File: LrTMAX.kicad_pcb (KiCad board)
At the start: 4 copper layers, 100 x 100 mm, 126 parts, among them J1 USB_C_Receptacle_USB2.0, J2 Conn_02x05_Odd_Even, Q1 2N7002, SW1 Tact_SW_8mm, SW10 EC11_SMD, SW11 EC11_SMD, SW12 EC11_SMD, SW13 EC11_SMD, SW14 EC11_SMD, SW15 EC11_SMD, SW16 EC11_SMD, SW17 EC11_SMD, SW2 Tact_SW_8mm, SW20 SW_SPST, SW3 Tact_SW_8mm, SW4 Tact_SW_8mm, SW5 Tact_SW_8mm, SW6 Tact_SW_8mm, SW7 Tact_SW_8mm, SW8 Tact_SW_8mm, U1 STM32F072C8Tx, U3 SSD1306_OLED_0.91, U4 SPX3819M5-L3-3TR

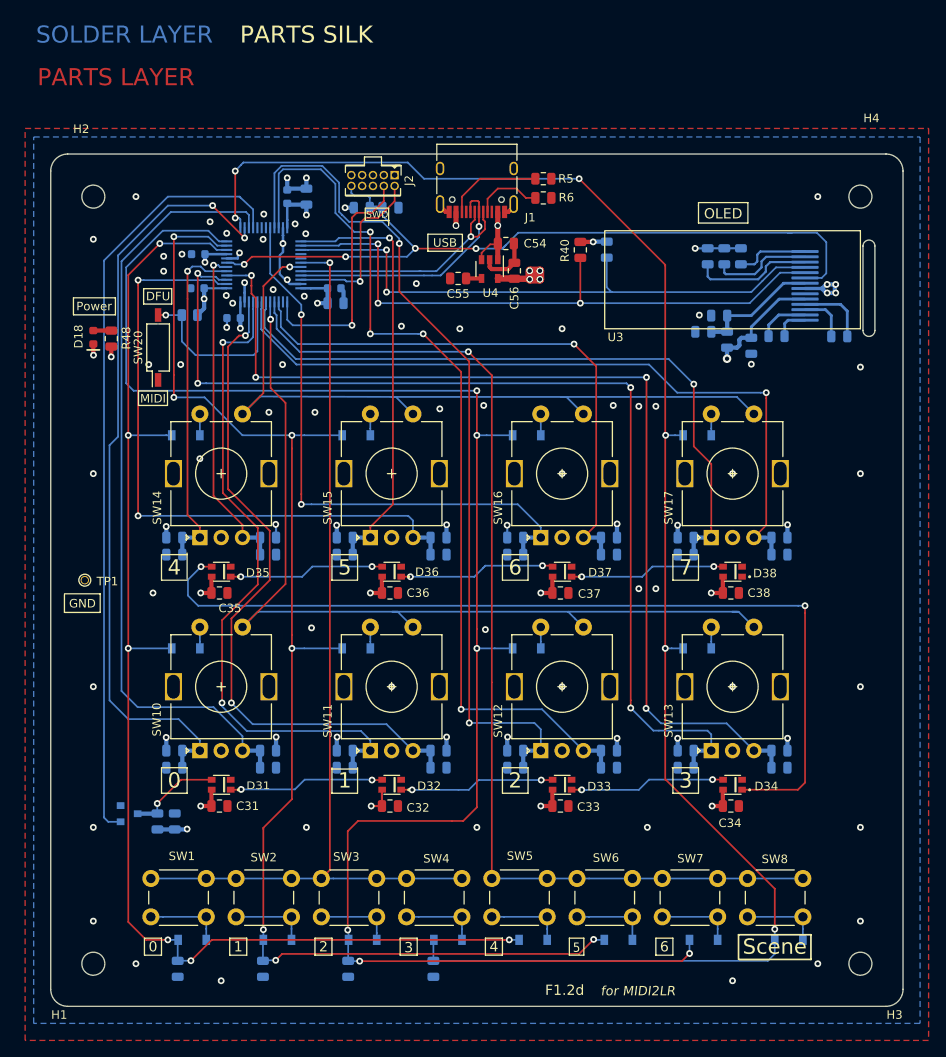
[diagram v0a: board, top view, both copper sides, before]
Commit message: trace drawn except CPU.
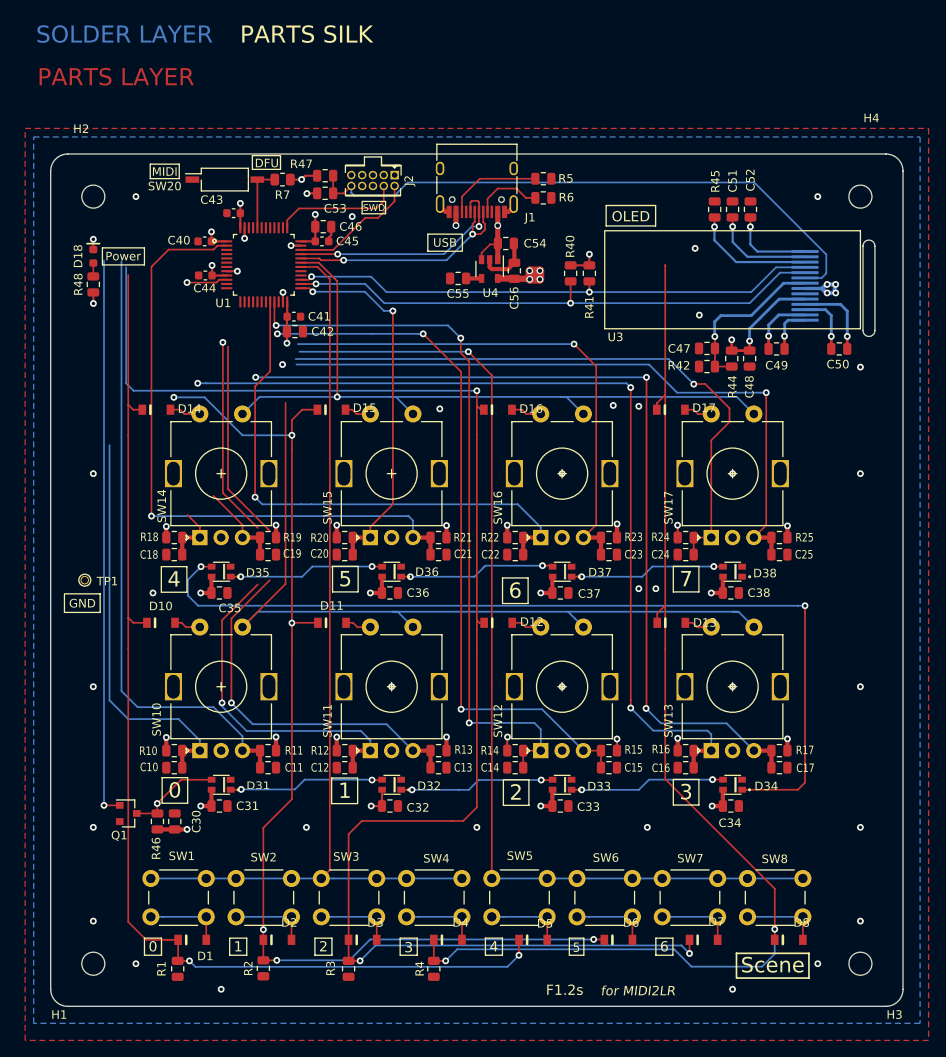
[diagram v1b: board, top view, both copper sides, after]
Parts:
- C10, C11, C12, C13, C14, C15, C16, C17, C18, C19, C20, C21, C22, C23, C24, C25, C30, C40, C41, C42, C43, C44, C45, C46, C47, C48, C49, C50, C51, C52, C53, D1, D10, D11, D12, D13, D14, D15, D16, D17, D2, D3, D4, D5, D6, D7, D8, Q1, R1, R10, R11, R12, R13, R14, R15, R16, R17, R18, R19, R2, R20, R21, R22, R23, R24, R25, R3, R4, R41, R42, R44, R45, R46, R47, R7, U1: moved to F.Cu
- moved SW20 21.2 mm to (120.4, 103.0), turned to 0 degrees
- moved R7 19.3 mm to (127.2, 103.0)
- moved C42 15.9 mm to (128.7, 120.8), turned to 180 degrees
- moved C41 14.1 mm to (128.5, 119.1), turned to 180 degrees
- moved C43 12.3 mm to (121.5, 106.9)
- moved D18 9.50 mm to (105.0, 112.0), turned to -90 degrees
- moved C46 9.08 mm to (132.0, 108.5)
- moved C53 7.85 mm to (132.2, 104.6), turned to 180 degrees
- moved R48 6.70 mm to (105.0, 115.3)
- moved R47 5.71 mm to (132.2, 102.5)
- moved C45 5.68 mm to (131.8, 110.2)
- moved C52 5.61 mm to (182.1, 106.5)
- moved C51 5.58 mm to (180.0, 106.5)
- moved C40 5.57 mm to (118.1, 110.2)
- moved R45 5.56 mm to (177.9, 106.5)
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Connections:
- net Net-(R7-Pad2) renamed /DFU
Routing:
- net /M3: track 196.4 -> 136.4 mm, vias 6 -> 2
- net /ENC0A: track 90.4 -> 47.7 mm, vias 2 -> 0
- net /ENC4A: track 41.0 -> 7.32 mm, vias 1 -> 0
- net /M1: track 157.2 -> 128.1 mm, vias 7 -> 6
- net /ENC4B: track 39.1 -> 10.4 mm, vias 1 -> 0
- net /LED_DON: track 90.9 -> 65.7 mm, vias 0 -> 1
- net /ENC2B: track 106.8 -> 83.4 mm, vias 4 -> 3
- net /NRST: track 92.3 -> 70.3 mm, vias 4 -> 0
- net /M2: track 200.1 -> 179.9 mm, vias 6 -> 3
- net /ENC0B: track 91.6 -> 72.6 mm
- net GND: track 45.8 -> 27.1 mm, vias 72 -> 43
- net /ENC3A: track 121.9 -> 105.3 mm, vias 4 -> 3
- net /ENC2A: track 102.4 -> 86.0 mm, vias 2 -> 3
- net /ENC3B: track 118.5 -> 103.5 mm, vias 4 -> 3
- net /ENC1A: track 78.4 -> 63.8 mm
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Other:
- board text added: "F1.2s"
- board text removed: "F1.2d"
